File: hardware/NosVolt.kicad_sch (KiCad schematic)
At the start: 10 parts, among them J101 INPUTS, J102 OUTPUTS, SW101 SW_Reset, SW102 SSSS811101, U101 ESP32-S3-WROOM-1

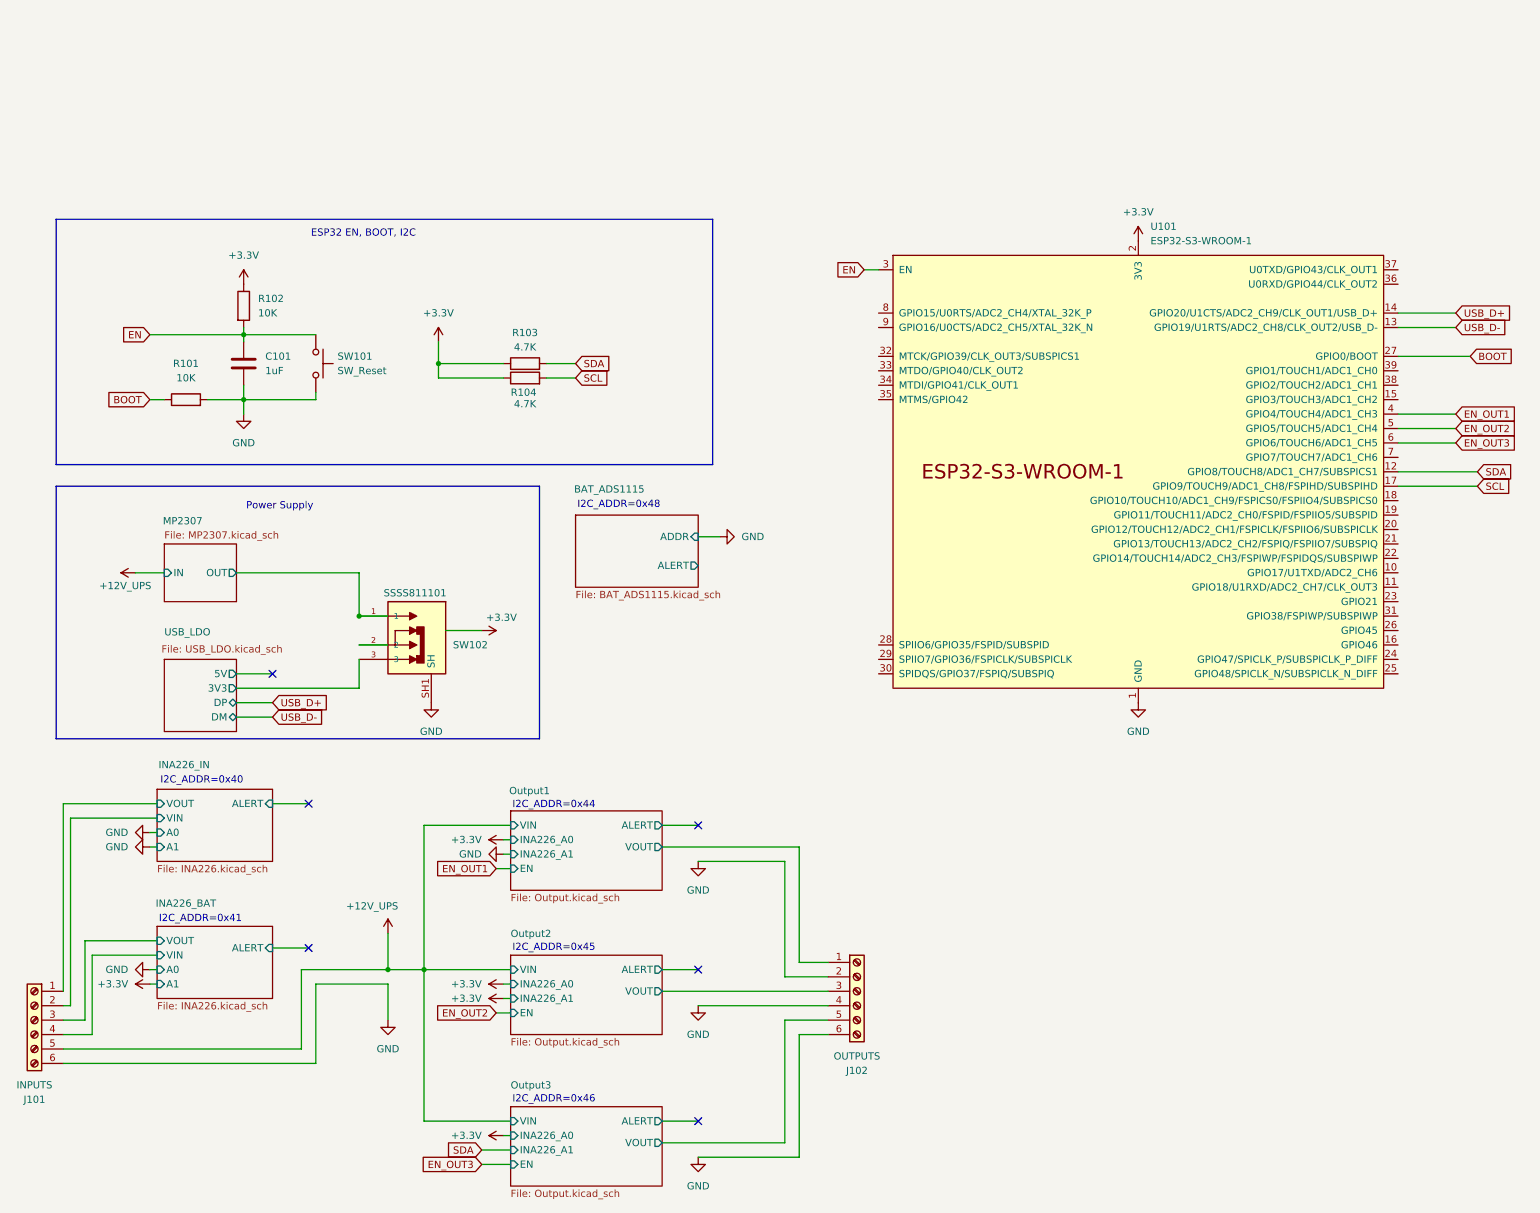
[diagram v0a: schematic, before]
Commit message: Add screen
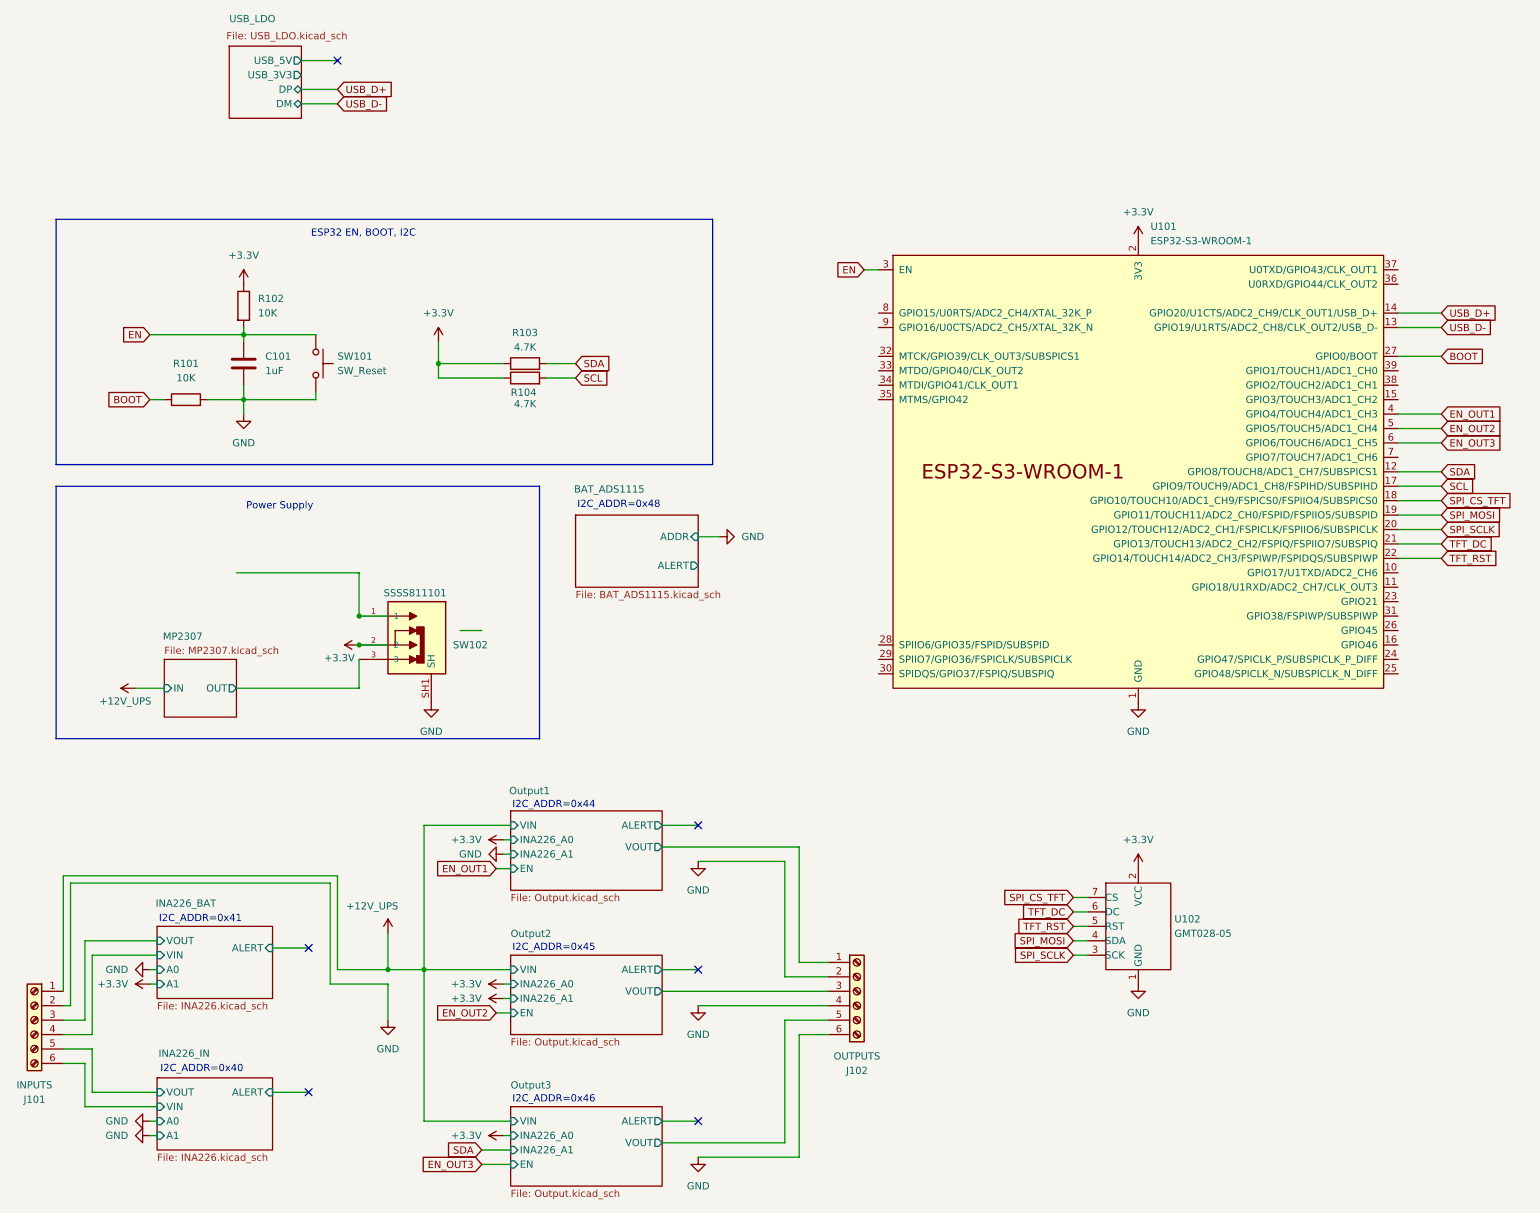
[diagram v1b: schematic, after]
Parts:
- added U102: GMT028-05, NosLib:GMT028-05, symbol NosLib:GMT028-05
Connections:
- net USB_LDO/3V3 is gone; now on net MP2307/OUT: SW102.3
- net +12V_UPS: now also J101.1 (Pin_1); no longer J101.5 (Pin_5)
- net +3.3V: now also SW102.2, U102.2 (VCC)
- net GND: now also J101.2 (Pin_2), U102.1 (GND); no longer J101.6 (Pin_6)
- net INA226_IN/VIN: now also J101.6 (Pin_6); no longer J101.2 (Pin_2)
- net INA226_IN/VOUT: now also J101.5 (Pin_5); no longer J101.1 (Pin_1)
- net MP2307/OUT: no longer SW102.1
- net SPI_CS_TFT: now reaches U101.18 (GPIO10/TOUCH10/ADC1_CH9/FSPICS0/FSPIIO4/SUBSPICS0)
- net SPI_CS_TFT: now also U102.7 (CS)
- net SPI_MOSI: now reaches U101.19 (GPIO11/TOUCH11/ADC2_CH0/FSPID/FSPIIO5/SUBSPID)
- net SPI_MOSI: now also U102.4 (SDA)
- net SPI_SCLK: now reaches U101.20 (GPIO12/TOUCH12/ADC2_CH1/FSPICLK/FSPIIO6/SUBSPICLK)
- net SPI_SCLK: now also U102.3 (SCK)
- net TFT_DC: now reaches U101.21 (GPIO13/TOUCH13/ADC2_CH2/FSPIQ/FSPIIO7/SUBSPIQ)
- net TFT_DC: now also U102.6 (DC)
- net TFT_RST: now reaches U101.22 (GPIO14/TOUCH14/ADC2_CH3/FSPIWP/FSPIDQS/SUBSPIWP)
- net TFT_RST: now also U102.5 (RST)
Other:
- sheet USB_LDO ports: added USB_3V3, USB_5V; removed 3V3, 5V
